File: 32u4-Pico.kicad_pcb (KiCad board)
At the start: 2 copper layers, 21.3 x 51.3 mm, 27 parts, among them J3 2.54mm header 01x20, J4 2.54mm header 01x20, U1 ATmega32U4-MU, Y1 8MHz 3225_4p crystal

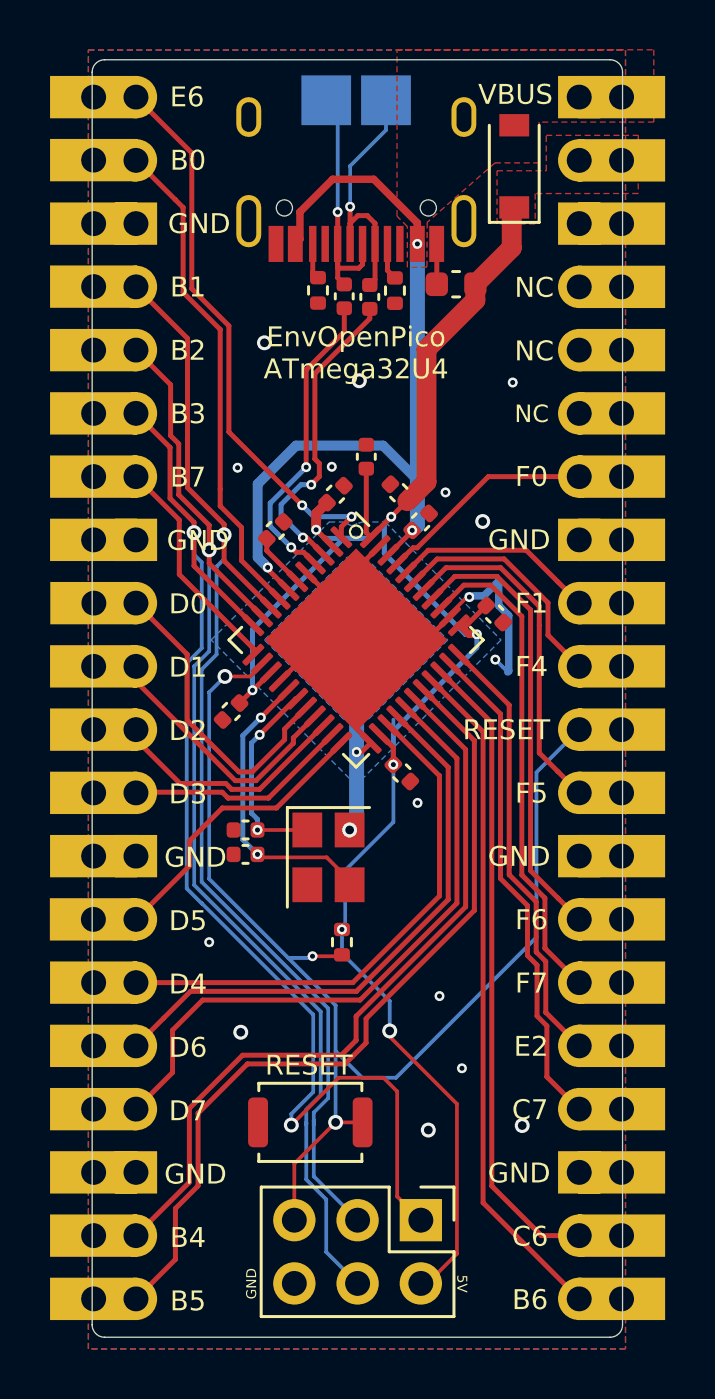
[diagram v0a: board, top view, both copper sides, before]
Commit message: smol fix-y
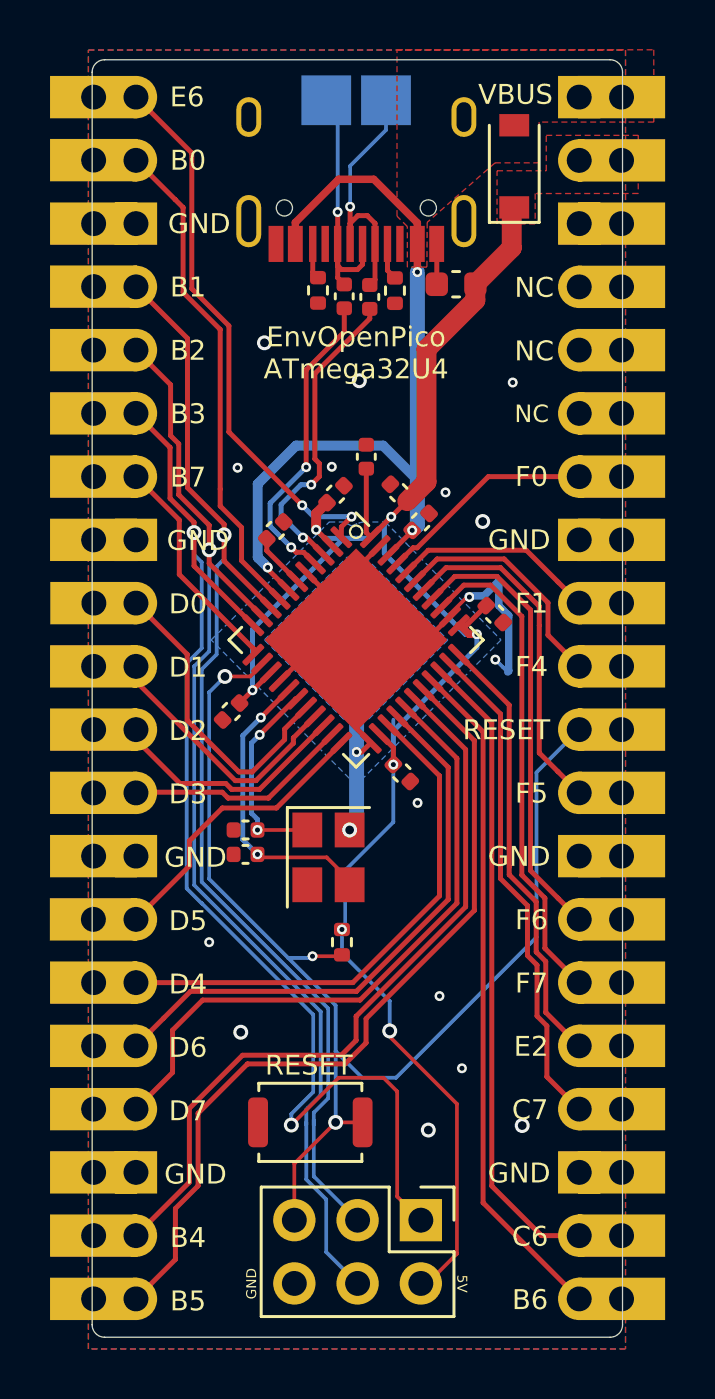
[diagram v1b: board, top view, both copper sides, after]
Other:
- net class Default removed
- net class USB_DIFF_90 removed
